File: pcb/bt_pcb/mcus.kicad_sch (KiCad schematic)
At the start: 38 parts, among them IC11 STM32H523CEU6, IC4 STM32H750VBT6, IC5 W25Q512JVEIM, J14 Conn_02x09_Top_Bottom, J15 Conn_JTAG_SWD_10, J2 Conn_JTAG_SWD_10, Y1 Crystal, Y2 Crystal

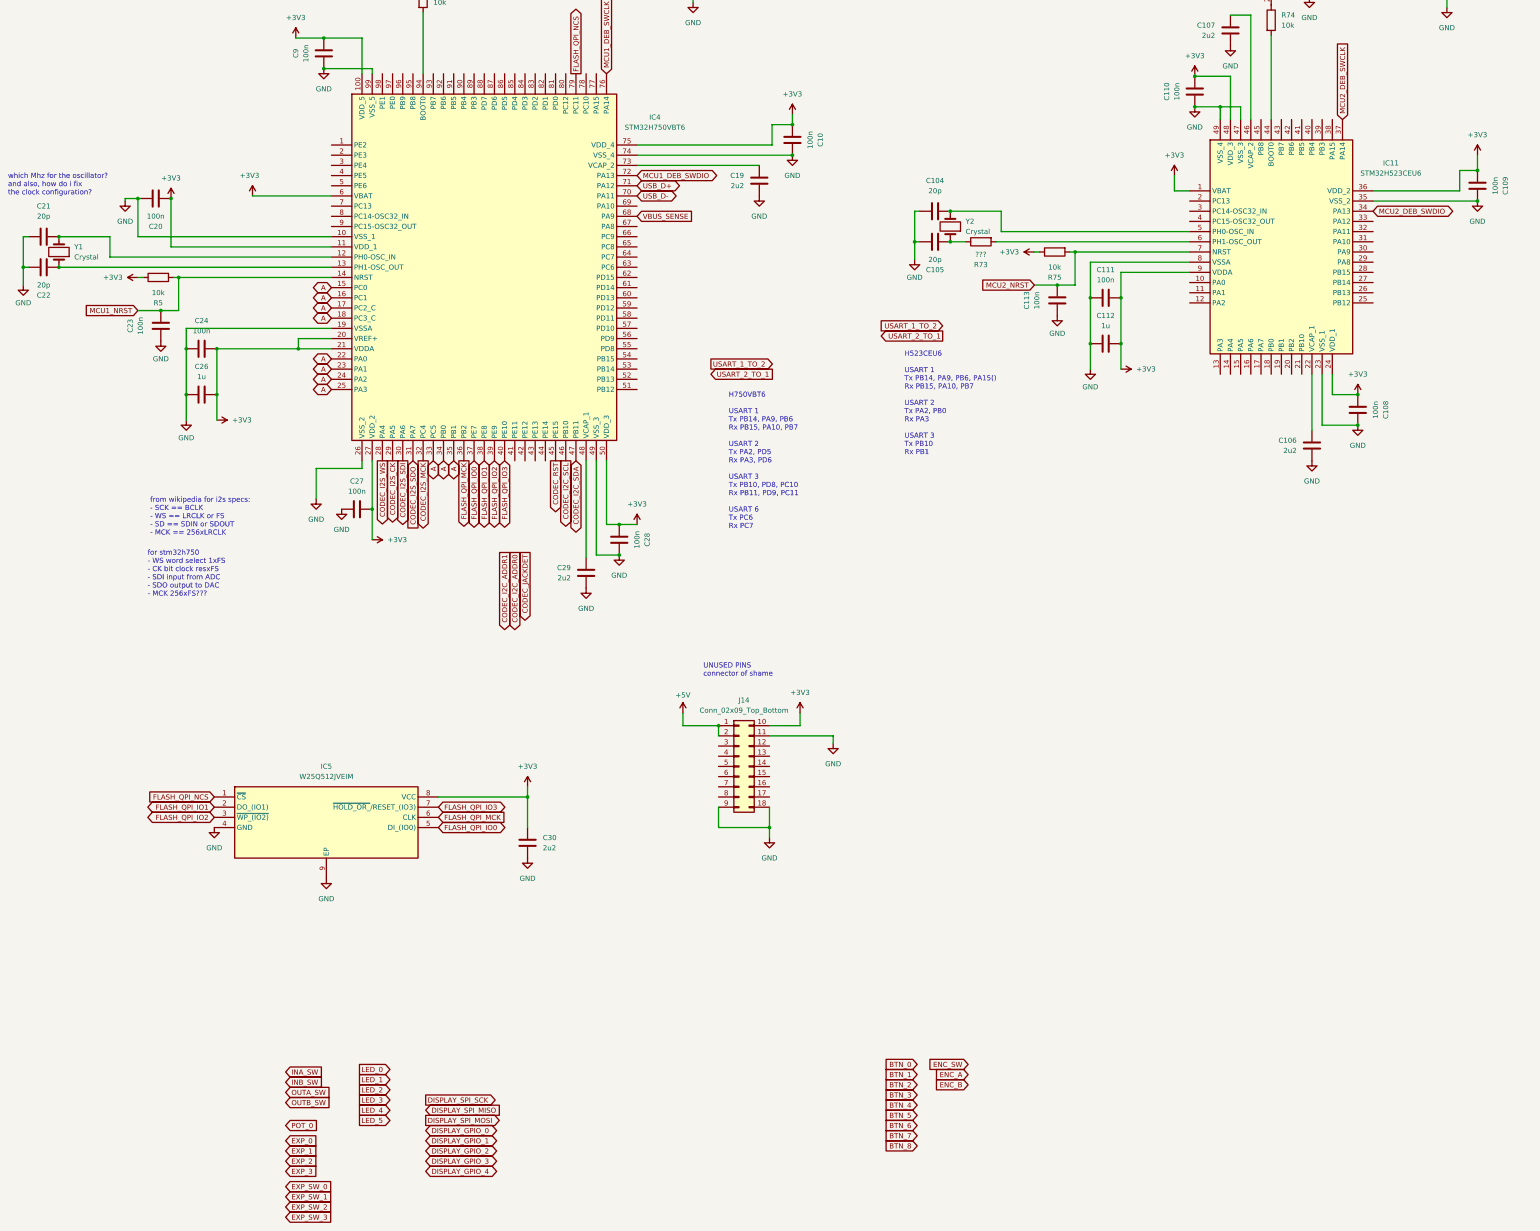
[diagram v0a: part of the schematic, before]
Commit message: big progress, now revising error and warnings
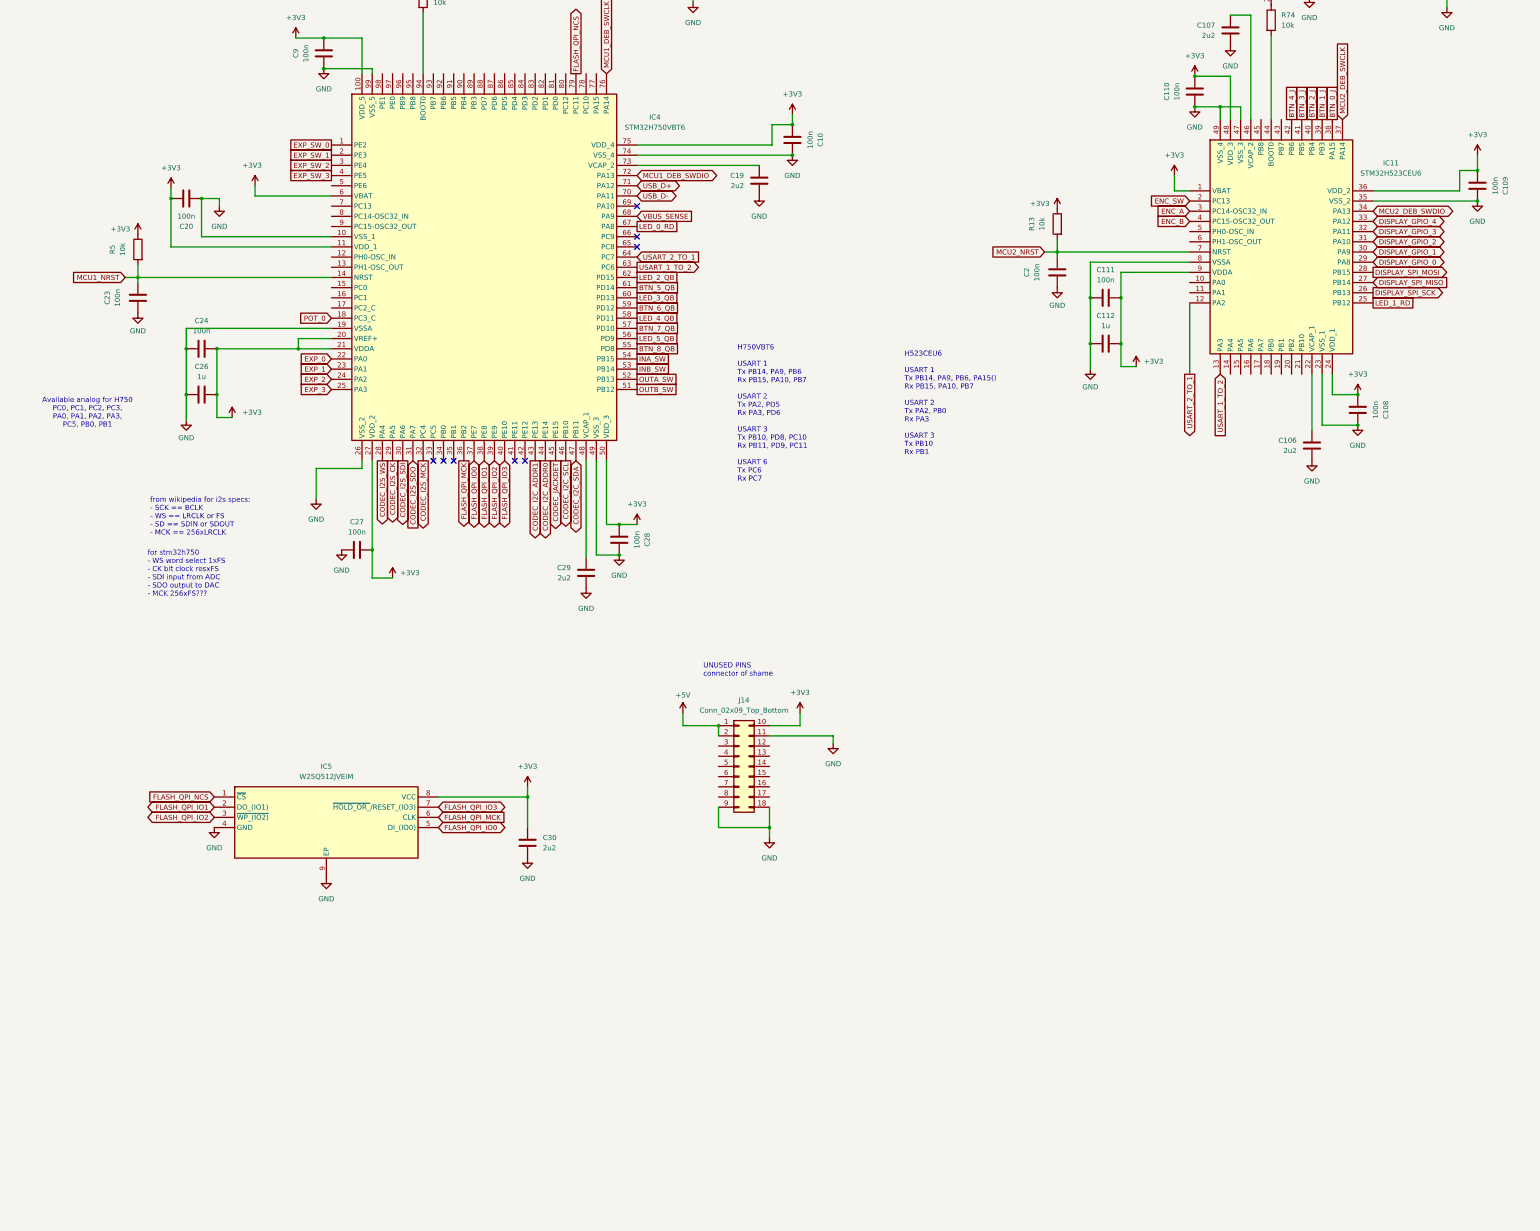
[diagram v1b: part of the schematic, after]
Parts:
- removed C104, C105, C21, C22: 20p, symbol Device:C
- removed C113: 100n, symbol Device:C
- removed R73: ???, symbol Device:R
- removed R75: 10k, symbol Device:R
- removed Y1, Y2: Crystal, symbol Device:Crystal
- added C2: 100n, symbol Device:C
- added R13: 10k, symbol Device:R
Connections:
- net CODEC_RST is gone; now on net CODEC_JACKDET: IC4.45 (PE15)
- net +3V3: now also C20.1, R13.1; no longer C20.2
- net CODEC_I2C_ADDR0: now also IC4.44 (PE14)
- net CODEC_I2C_ADDR1: now also IC4.43 (PE13)
- net DISPLAY_GPIO_0: now also IC11.29 (PA8)
- net DISPLAY_GPIO_1: now also IC11.30 (PA9)
- net DISPLAY_GPIO_2: now also IC11.31 (PA10)
- net DISPLAY_GPIO_3: now also IC11.32 (PA11)
- net DISPLAY_GPIO_4: now also IC11.33 (PA12)
- net DISPLAY_SPI_MISO: now also IC11.27 (PB14)
- net DISPLAY_SPI_MOSI: now also IC11.28 (PB15)
- net DISPLAY_SPI_SCK: now also IC11.26 (PB13)
- net ENC_A: now also IC11.3 (PC14-OSC32_IN)
- net ENC_B: now also IC11.4 (PC15-OSC32_OUT)
- net ENC_SW: now also IC11.2 (PC13)
- net EXP_0: now also IC4.22 (PA0)
- net EXP_1: now also IC4.23 (PA1)
- net EXP_2: now also IC4.24 (PA2)
- net EXP_3: now also IC4.25 (PA3)
- net EXP_SW_0: now also IC4.1 (PE2)
- net EXP_SW_1: now also IC4.2 (PE3)
- net EXP_SW_2: now also IC4.3 (PE4)
- net EXP_SW_3: now also IC4.4 (PE5)
- net GND: now also C20.2, C2.1; no longer C20.1
- net INA_SW: now also IC4.54 (PB15)
- net INB_SW: now also IC4.53 (PB14)
- net MCU2_NRST: now also C2.2, R13.2
- net OUTA_SW: now also IC4.52 (PB13)
- net OUTB_SW: now also IC4.51 (PB12)
- net POT_0: now also IC4.18 (PC3_C)
- net USART_1_TO_2: now also IC11.13 (PA3), IC4.63 (PC6)
- net USART_2_TO_1: now also IC11.12 (PA2), IC4.64 (PC7)
- net LED_1_RD: now reaches IC11.25 (PB12)
- net BTN_0_J: now reaches IC11.38 (PA15)
- net BTN_1_J: now reaches IC11.39 (PB3)
- net BTN_2_J: now reaches IC11.40 (PB4)
- net BTN_3_J: now reaches IC11.41 (PB5)
- net BTN_4_J: now reaches IC11.42 (PB6)
- net BTN_8_QB: now reaches IC4.55 (PD8)
- net LED_5_QB: now reaches IC4.56 (PD9)
- net BTN_7_QB: now reaches IC4.57 (PD10)
- net LED_4_QB: now reaches IC4.58 (PD11)
- net BTN_6_QB: now reaches IC4.59 (PD12)
- net LED_3_QB: now reaches IC4.60 (PD13)
- net BTN_5_QB: now reaches IC4.61 (PD14)
- net LED_2_QB: now reaches IC4.62 (PD15)
- net LED_0_RD: now reaches IC4.67 (PA8)
- removed net A: IC4.15 (PC0), IC4.16 (PC1), IC4.17 (PC2_C), IC4.18 (PC3_C), IC4.22 (PA0), IC4.23 (PA1), IC4.24 (PA2), IC4.25 (PA3), IC4.33 (PC5), IC4.34 (PB0), IC4.35 (PB1)
- no-connect marks 4 -> 12
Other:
- note added: "Available analog for H750 PC0, PC1, PC2, PC3, PA0, PA1, PA2, PA3, PC5, PB0, PB1"
- note removed: "which Mhz for the oscillator? and also, how do i fix the clock configuration?"
- moved on the sheet: C20, C23, C27, R5

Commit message: solving some erc warnings and errors
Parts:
- renumbered C23 to C43, C20 to C44, C24 to C45, C26 to C46, C9 to C47, C27 to C48, C30 to C49, C29 to C50, C28 to C51, C19 to C52, C10 to C53, C2 to C54, C111 to C55, C112 to C56, C110 to C57, C107 to C58, C106 to C59, C108 to C60, C109 to C61, IC5 to IC3, IC11 to IC5, J2 to J12, J14 to J13, J15 to J14, JP2 to JP3, JP1 to JP4, R5 to R35, R3 to R36, R13 to R37, R74 to R38
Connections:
- net +5V: no longer J13.2 (Pin_2)
- net GND: now also J13.2 (Pin_2); no longer J13.18 (Pin_18), J13.9 (Pin_9)
- no-connect marks 12 -> 4
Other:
- moved on the sheet: C43, C44, C48, C50, C51, C52, C55, C56, C57, C58, C61, IC3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
